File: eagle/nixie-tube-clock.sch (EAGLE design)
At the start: 88 parts, among them IC1 HV5622QC, IC2 HV5622QC, IC3 LM555D, IC5 LD117ADT33TR, P1 1 k, Q1 BC817-25SMD, Q2 BC817-25SMD, Q3 BC817-25SMD, Q4 BC817-25SMD, T1 BC547B, T2 TK3P50D, T3 BST51, T4 BST51, T5 BST51

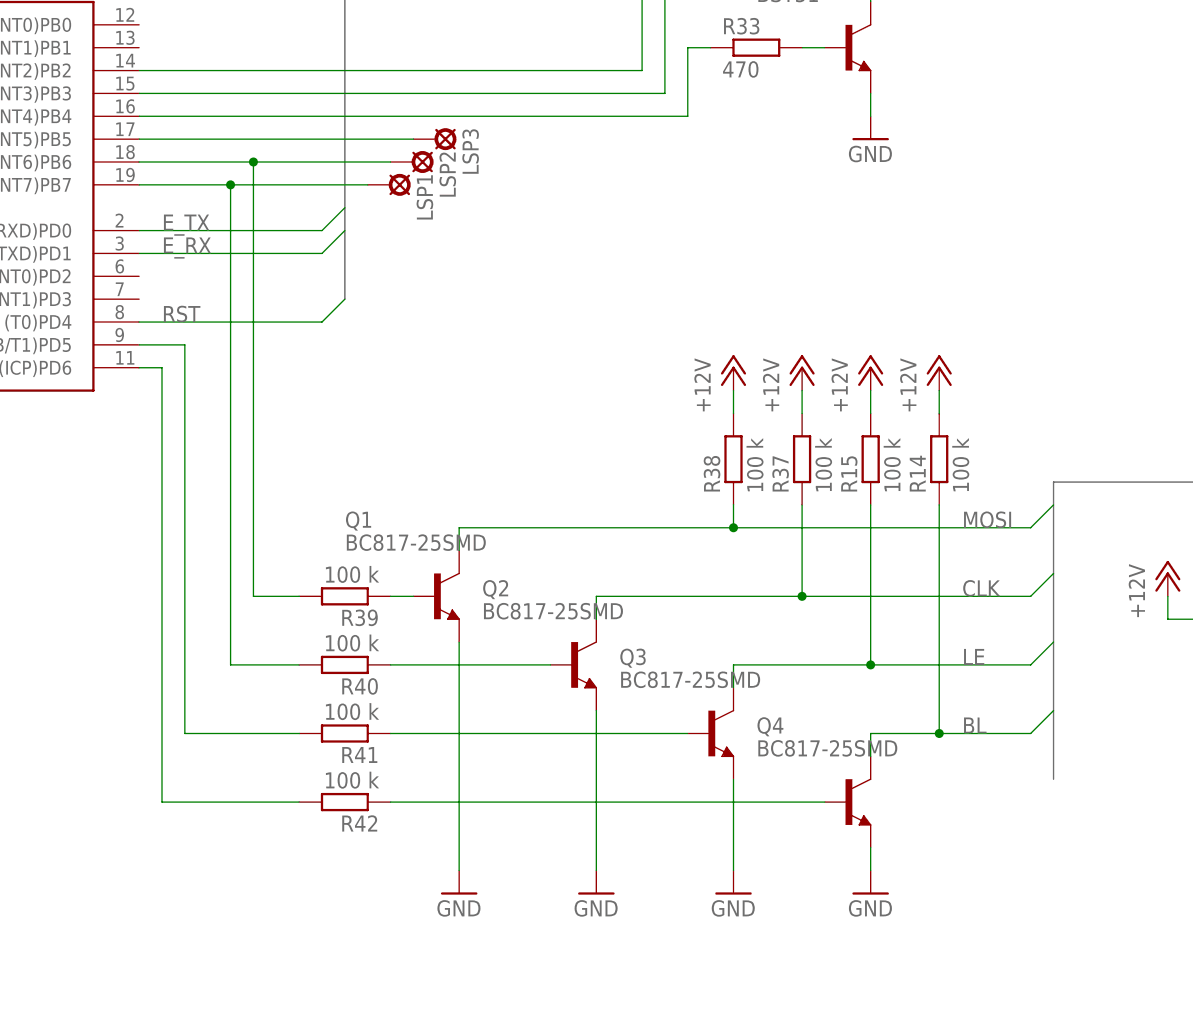
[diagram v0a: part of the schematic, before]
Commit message: Alfa v2 version of schematic
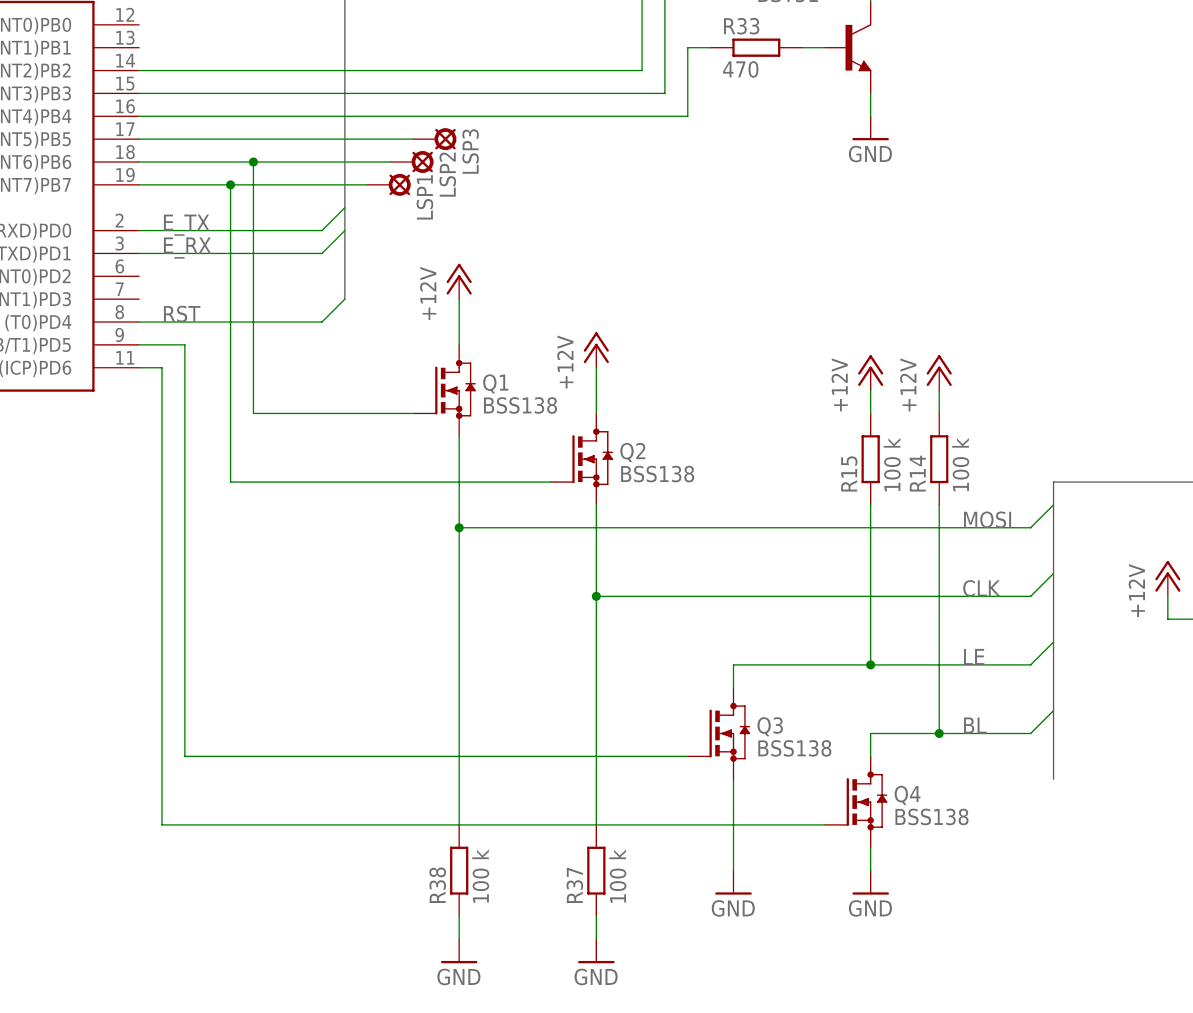
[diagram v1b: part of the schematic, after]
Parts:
- removed R39, R40, R41, R42: 100 k, resistor:R-EU_R1206
- Q1, Q2, Q3, Q4: value BC817-25SMD -> BSS138; device transistor-npn:BC817-25SMD -> transistor-small-signal:BSS123
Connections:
- removed net N$1: Q1.B, R39.1
- removed net N$17: Q3.B, R41.1
- removed net N$2: Q2.B, R40.1
- removed net N$31: Q4.B, R42.1
- net +12V: now also Q1.D, Q2.D; no longer R37.2, R38.2
- net BL: now also Q4.D; no longer Q4.C
- net CLK: now also Q2.S, R37.2; no longer Q2.C, R37.1
- net GND: now also Q3.S, Q4.S, R37.1, R38.1; no longer Q1.E, Q2.E, Q3.E, Q4.E
- net LE: now also Q3.D; no longer Q3.C
- net MOSI: now also Q1.S, R38.2; no longer Q1.C, R38.1
- net N$19: now also Q4.G; no longer R42.2
- net N$23: now also Q1.G; no longer R39.2
- net N$25: now also Q2.G; no longer R40.2
- net N$29: now also Q3.G; no longer R41.2
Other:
- moved on the sheet: R37, R38

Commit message: Beta version of schematic
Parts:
- removed LSP1: SCL, solpad:SE11
- removed LSP2: MISO, solpad:SE11
- removed LSP3: MOSI, solpad:SE11
- removed LSP4: VCC, solpad:SE11
- removed LSP5: RST, solpad:SE11
- removed Q2, Q3: BSS138, transistor-small-signal:BSS123
- removed R32, R33, R34: 470, resistor:R-EU_R1206
- removed U$1: TINY2313, atmel:TINY2313
- removed X4: (no value), con-ptr500:AK300/2
- added +: +, testpad:TPPAD1-17
- added -: -, testpad:TPPAD1-17
- added C8, C9: 22 pF, resistor:C-EUC1206
- added IC4: MEGA8-AI, atmel:MEGA8-AI
- added MISO: MISO, solpad:SE11
- added MOSI: MOSI, solpad:SE11
- added RST: RST, solpad:SE11
- added SCK: SCK, solpad:SE11
- added T7, T8, T9: IRLL014NTRPBF, transistor-fet:IRLL014NTRPBF
- added VCC: VCC, solpad:SE11
- C1: value 47 uF / 16 V -> 100 uF / 16 V
- D1: value GF1 -> 1A 600V
- Q1: value BSS138 -> 8 MHz; device transistor-small-signal:BSS123 -> crystal:CRYSTALHC49S
- R13, R46: value 270 -> 330k
- R16, R17, R19, R20, R22, R23, R25, R26: value 150 -> 270
- R18, R21, R24, R27: value 180 -> 330
- T3, T4, T5: value BST51 -> BSS138; device transistor:-NPN-SOT89-BCE -> transistor-small-signal:BSS123
- renumbered D2 to D1, Q4 to T6
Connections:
- removed net N$135: R34.2, T5.B
- removed net N$136: R32.2, T3.B
- removed net N$137: R33.2, T4.B
- removed net N$24: LED2-B.C
- removed net N$30: LED3-B.C
- removed net N$35: LSP5.MP, U$1.PA2(RESET/DW)
- removed net N$36: LED4-B.C
- removed net N$37: LSP3.MP, U$1.(MOSI/DI/SDA/PCINT5)PB5
- removed net N$42: LED5-B.C
- removed net N$48: LED6-B.C
- removed net N$54: LED7-B.C
- new net N$1: IC4.PC6(/RESET), RST.MP
- new net N$17: IC4.PB4(MISO), MISO.MP
- new net N$2: IC4.PB3(MOSI/OC2), MOSI.MP, T3.G
- new net N$31: C9.1, IC4.PB6(XTAL1/TOSC1), Q1.1
- net +12V: now also +.TP, T3.D, T4.D; no longer Q1.D, Q2.D, X4-1.KL
- net +3V3: now also IC4.AVCC, IC4.VCC@1, IC4.VCC@2, VCC.MP; no longer LSP4.MP, U$1.VCC
- net CLK: now also T4.S; no longer Q2.S
- net E_RX: now also IC4.PD1(TXD); no longer U$1.(TXD)PD1
- net E_TX: now also IC4.PD0(RXD); no longer U$1.(RXD)PD0
- net GND: now also -.TP, C8.2, C9.2, IC4.GND, IC4.GND@1, IC4.GND@2, T5.S, T7.S, T8.S, T9.S; no longer Q3.S, T3.E, T4.E, T5.E, U$1.GND, X4-2.KL
- net LE: now also T5.D; no longer Q3.D
- net LED_B: now also LED2-B.C, LED3-B.C, LED4-B.C, LED5-B.C, LED6-B.C, LED7-B.C, T7.D; no longer T4.C
- net LED_D0: now also IC4.PC0(ADC0), T9.G; no longer R34.1, U$1.(OC0A/PCINT2)PB2
- net LED_D1: now also IC4.PC1(ADC1), T8.G; no longer R32.1, U$1.(OC1A/PCINT3)PB3
- net LED_D2: now also IC4.PC2(ADC2), T7.G; no longer R33.1, U$1.(OC1B/PCINT4)PB4
- net LED_G: now also T8.D; no longer T3.C
- net LED_R: now also T9.D; no longer T5.C
- net MIN_1_0: now also IC2.HVOUT23; no longer IC2.HVOUT22, IC2.HVOUT32
- net MIN_1_1: now also IC2.HVOUT24; no longer IC2.HVOUT23
- net MIN_1_2: now also IC2.HVOUT25; no longer IC2.HVOUT24
- net MIN_1_3: now also IC2.HVOUT26; no longer IC2.HVOUT25
- net MIN_1_4: now also IC2.HVOUT27; no longer IC2.HVOUT26
- net MIN_1_5: now also IC2.HVOUT28; no longer IC2.HVOUT27
- net MIN_1_6: now also IC2.HVOUT29; no longer IC2.HVOUT28
- net MIN_1_7: now also IC2.HVOUT30; no longer IC2.HVOUT29
- net MIN_1_8: now also IC2.HVOUT31; no longer IC2.HVOUT30
- net MIN_1_9: now also IC2.HVOUT32; no longer IC2.HVOUT31
- net MOSI: now also T3.S; no longer Q1.S
- net N$19: now also IC4.PB1(OC1A); no longer U$1.(ICP)PD6
- net N$23: now also C8.1, IC4.PB7(XTAL2/TOSC2), Q1.2; no longer LSP2.MP, Q1.G, U$1.(MISO/DO/PCINT6)PB6
- net N$25: now also IC4.PB5(SCK), SCK.MP, T4.G; no longer LSP1.MP, Q2.G, U$1.(UCSK/SCL/PCINT7)PB7
- net N$29: now also IC4.PB0(ICP), T5.G; no longer Q3.G, U$1.(OC0B/T1)PD5
- net RST: now also IC4.PD2(INT0); no longer U$1.(T0)PD4
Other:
- moved on the sheet: R37, R38
